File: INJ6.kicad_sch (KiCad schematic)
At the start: 9 parts, among them U10 VNLD5160TR-E, U11 VNLD5160TR-E, U9 VNLD5160TR-E

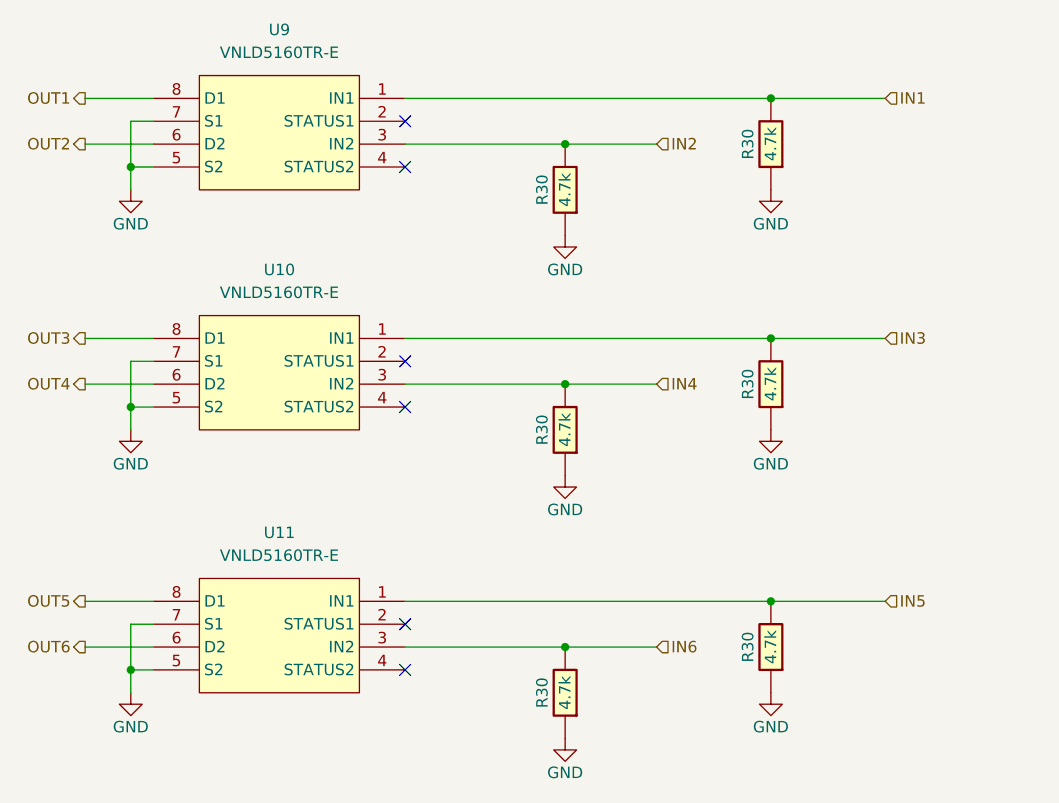
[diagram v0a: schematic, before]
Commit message: Unification with UAEFI F7 #114 #110
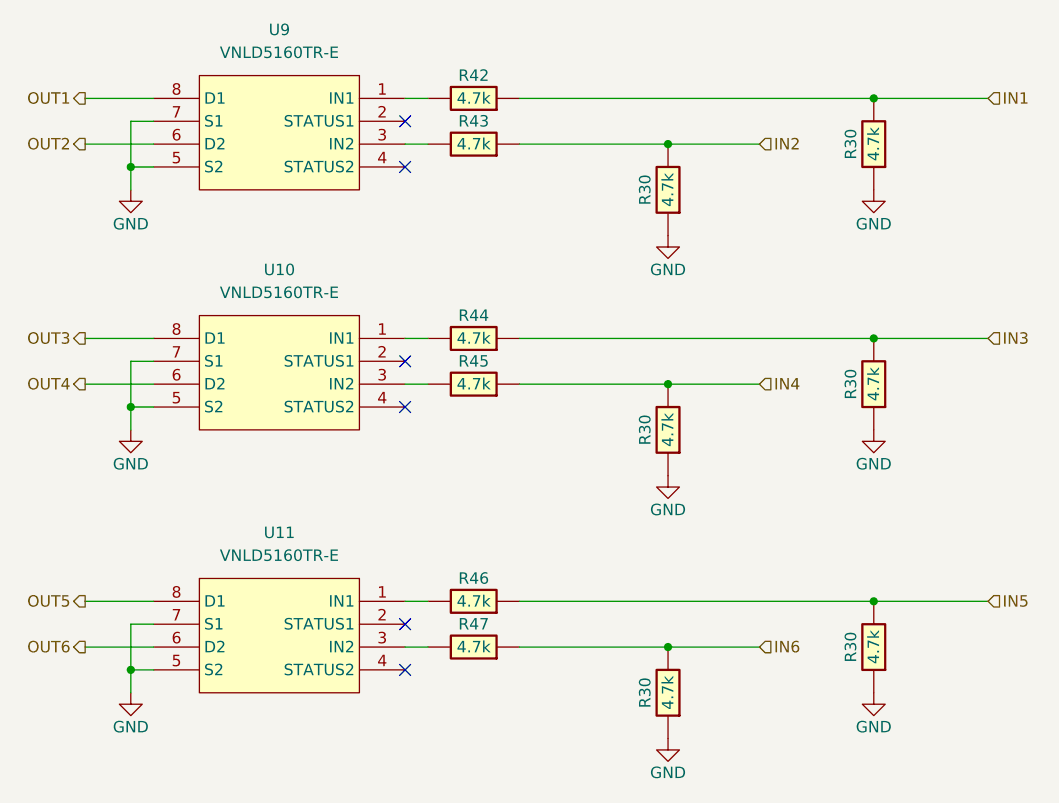
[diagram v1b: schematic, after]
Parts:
- added R42, R43, R44, R45, R46, R47: 4.7k, hellen-one-common:R0603, symbol hellen-one-common:Res
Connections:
- net IN1: now also R42.1; no longer U9.1 (IN1)
- net IN2: now also R43.1; no longer U9.3 (IN2)
- net IN3: now also R44.1; no longer U10.1 (IN1)
- net IN4: now also R45.1; no longer U10.3 (IN2)
- net IN5: now also R46.1; no longer U11.1 (IN1)
- net IN6: now also R47.1; no longer U11.3 (IN2)
- new net: R42.2, U9.1 (IN1)
- new net: R43.2, U9.3 (IN2)
- new net: R45.2, U10.3 (IN2)
- new net: R44.2, U10.1 (IN1)
- new net: R47.2, U11.3 (IN2)
- new net: R46.2, U11.1 (IN1)
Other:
- moved on the sheet: R30
